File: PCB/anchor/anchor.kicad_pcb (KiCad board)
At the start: 2 copper layers, 63.2 x 34.3 mm, 36 parts, among them J1 TSM-102-01-X-SV, J2 Conn_ARM_JTAG_SWD_10, J3 S2B-PH-SM4-TB_LF__SN_, J4 TSM-102-01-X-SV, J5 TSM-102-01-X-SV, J7 TSM-102-01-X-SV, J8 TSM-102-01-X-SV, Q1 IRLML2402TRPBF, Q2 IRLML2402TRPBF, U1 Voltage Regulator, U2 `, U3 LYR998

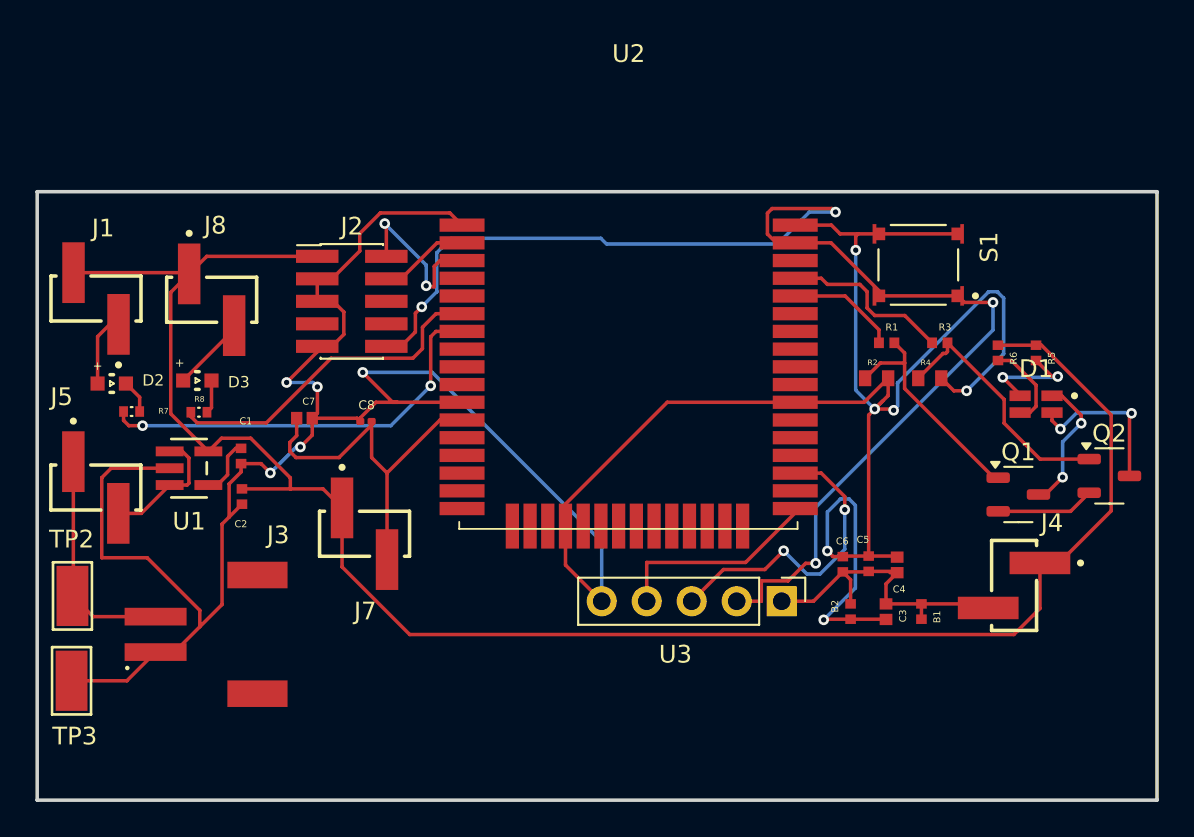
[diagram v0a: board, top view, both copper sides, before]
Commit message: anchor PCB v1
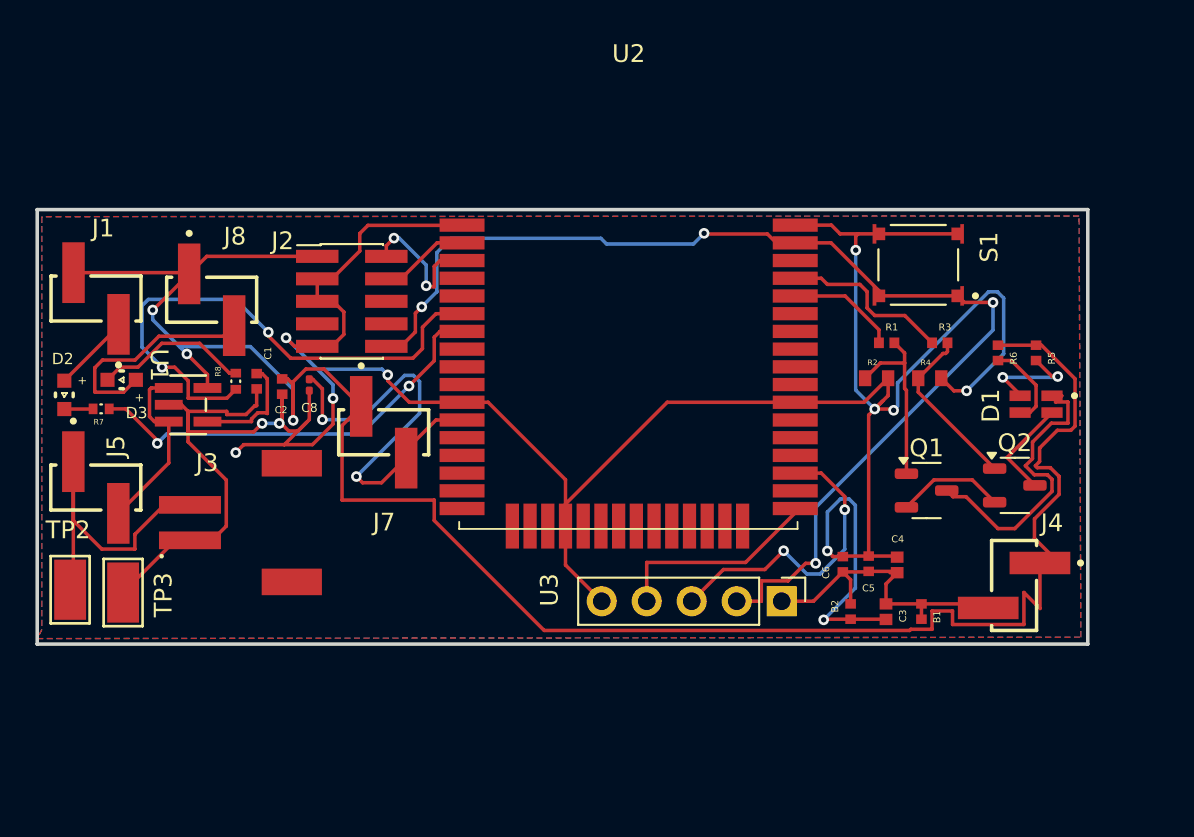
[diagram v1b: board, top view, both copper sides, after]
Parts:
- removed C7: 10uF, GRM155R60J106ME05D:CAPC1005X70N
- moved C2 6.61 mm to (155.4, 80.5)
- moved J3 6.60 mm to (150.2, 88.2)
- moved J7 5.83 mm to (161.2, 83.0)
- moved TP3 5.77 mm to (146.5, 92.1)
- moved Q2 5.36 mm to (196.8, 86.0)
- moved Q1 5.18 mm to (191.8, 86.3)
- moved C1 4.31 mm to (154.0, 80.2)
- moved D3 4.27 mm to (146.4, 80.1), turned to 0 degrees
- moved C8 3.81 mm to (157.0, 80.4), turned to -90 degrees
- moved U1 3.58 mm to (150.1, 81.5)
- moved D2 2.76 mm to (143.1, 80.9), turned to 90 degrees
- moved R8 2.72 mm to (152.8, 80.2), turned to -90 degrees
- moved R7 1.73 mm to (145.2, 81.7), turned to 0 degrees
- moved TP2 0.37 mm to (143.5, 91.9)
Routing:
- net Vreg +3.3V: track 104.3 -> 117.5 mm, vias 0 -> 3
- net Net-(U2-P0.17): track 19.0 -> 31.1 mm, vias 0 -> 2
- net GND: track 194.0 -> 183.3 mm, vias 11 -> 12
- net /RST: track 75.3 -> 65.8 mm
- net Net-(D1-K2): track 7.81 -> 17.1 mm, vias 2 -> 0
- net Net-(D3-A): track 4.29 -> 12.8 mm
- net Net-(D3-K): track 1.90 -> 8.79 mm
- net Net-(J3-Pad2): track 12.8 -> 19.4 mm
- net Net-(Q2-G): track 14.3 -> 9.66 mm
- net Net-(D1-K1): track 9.12 -> 5.81 mm, vias 2 -> 0
- net Net-(U1-NR): track 3.31 -> 6.37 mm
- net Vbatt +3.7V: track 7.36 -> 10.2 mm
- net Net-(U2-VDD): track 21.4 -> 24.2 mm, vias 0 -> 2
- net Net-(Q1-G): track 12.8 -> 10.3 mm
- net /SWD_DIO (BIDIRECTIONAL): track 9.70 -> 8.16 mm
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- added copper zone on B.Cu, net GND
- added copper zone on F.Cu, net GND
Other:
- board size 63.2 x 34.3 mm -> 59.3 x 24.5 mm
- rule pad_to_mask_clearance: 0 -> 0.0508
